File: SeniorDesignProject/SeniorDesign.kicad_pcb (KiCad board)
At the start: 2 copper layers, 32 parts, among them J1 RJ45(LoadCells), J2 RJ45(Accelerometer), J3 PICkit3, J5 ID-12LA Header, J6 XBEE Header, J7 7-Segment Display, P7 Power 1, U1 INA827, U2 LM1117-3.3, U3 ICL7660, U9 7805

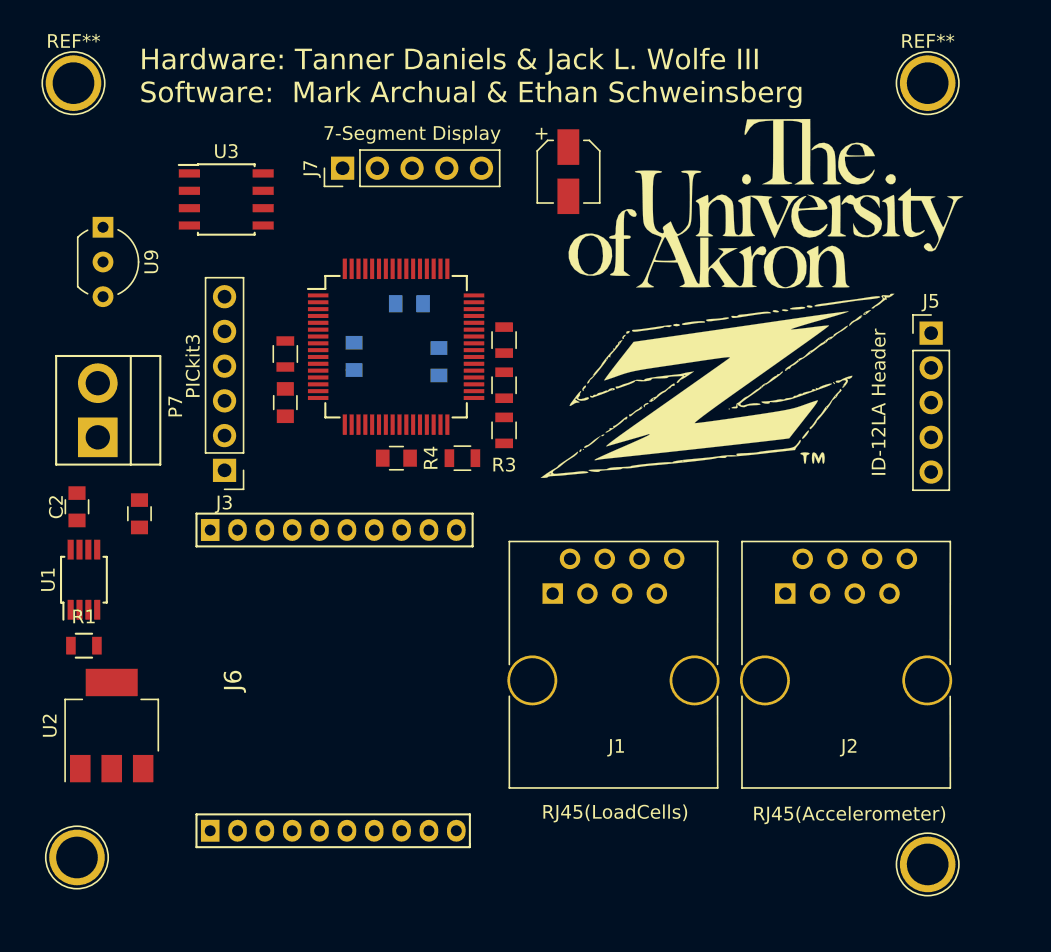
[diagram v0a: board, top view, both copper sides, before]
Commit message: Made more changes to board design and layout
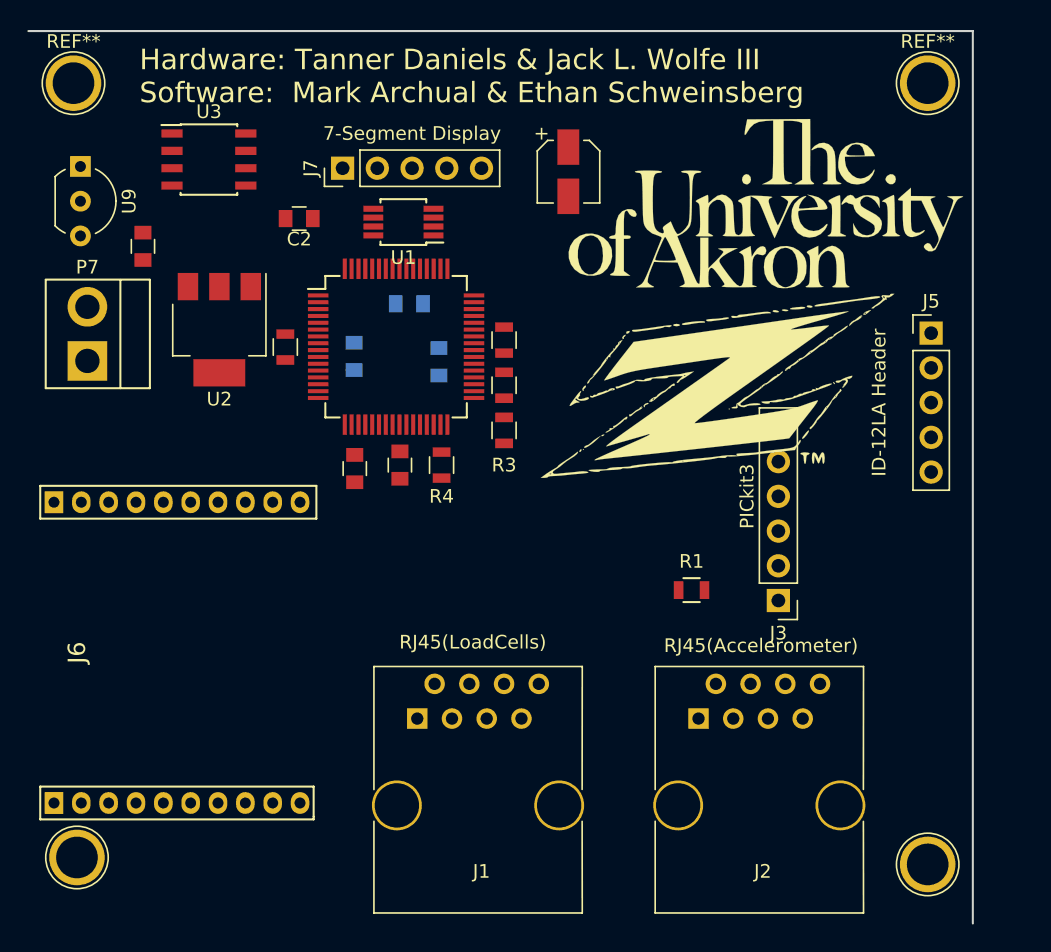
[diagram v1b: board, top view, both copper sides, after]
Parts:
- moved R1 44.6 mm to (165.4, 97.3)
- moved J3 41.6 mm to (171.7, 98.0)
- moved U1 35.1 mm to (144.3, 70.4), turned to 180 degrees
- moved U2 30.0 mm to (130.8, 78.2), turned to 270 degrees
- moved C2 26.6 mm to (136.7, 70.1), turned to 180 degrees
- moved C1 19.6 mm to (125.2, 72.1)
- moved J1 13.5 mm to (145.3, 106.7)
- moved J6 11.6 mm to (127.5, 101.9)
- moved J2 11.1 mm to (165.9, 106.7)
- moved C4 7.01 mm to (140.7, 88.4), turned to 90 degrees
- moved P7 5.64 mm to (121.2, 80.5)
- moved U9 4.74 mm to (120.7, 66.3)
- moved U3 3.19 mm to (130.0, 65.8)
- moved R4 1.61 mm to (147.1, 88.1), turned to 90 degrees
- moved C3 0.57 mm to (144.0, 88.1), turned to 270 degrees
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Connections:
- C2 pad 2: Net-(C2-Pad2) -> GND
- U9 pad 1: (no net) -> +5V
- U9 pad 2: (no net) -> GND
- U9 pad 3: (no net) -> +9V
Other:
- board outline added: 69.1 x 65.3 mm
